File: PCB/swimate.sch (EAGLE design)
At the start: 46 parts, among them IC1 LPC11U24, T1 BSS84, T2 BSS84, U1 USD-SOCKETNEW, U5 DS3231MZ/V+T, U6 MAX1595EUA33+, U7 MAX1811ESA-T, U8 MAX16054AZT+T, U9 HC_05, Y1 12.000MHz

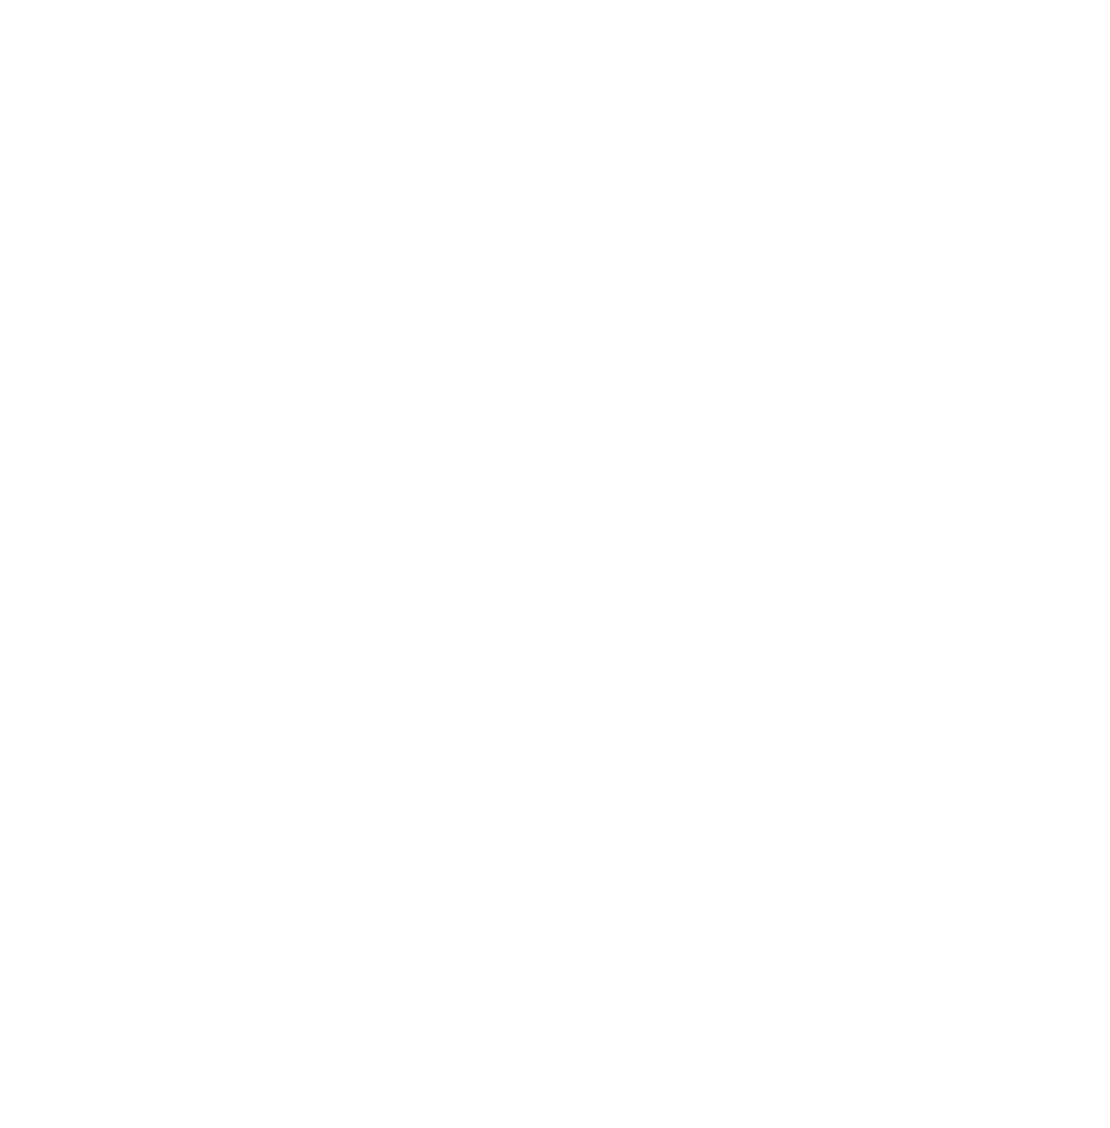
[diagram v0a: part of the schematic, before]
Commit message: Added dispaly
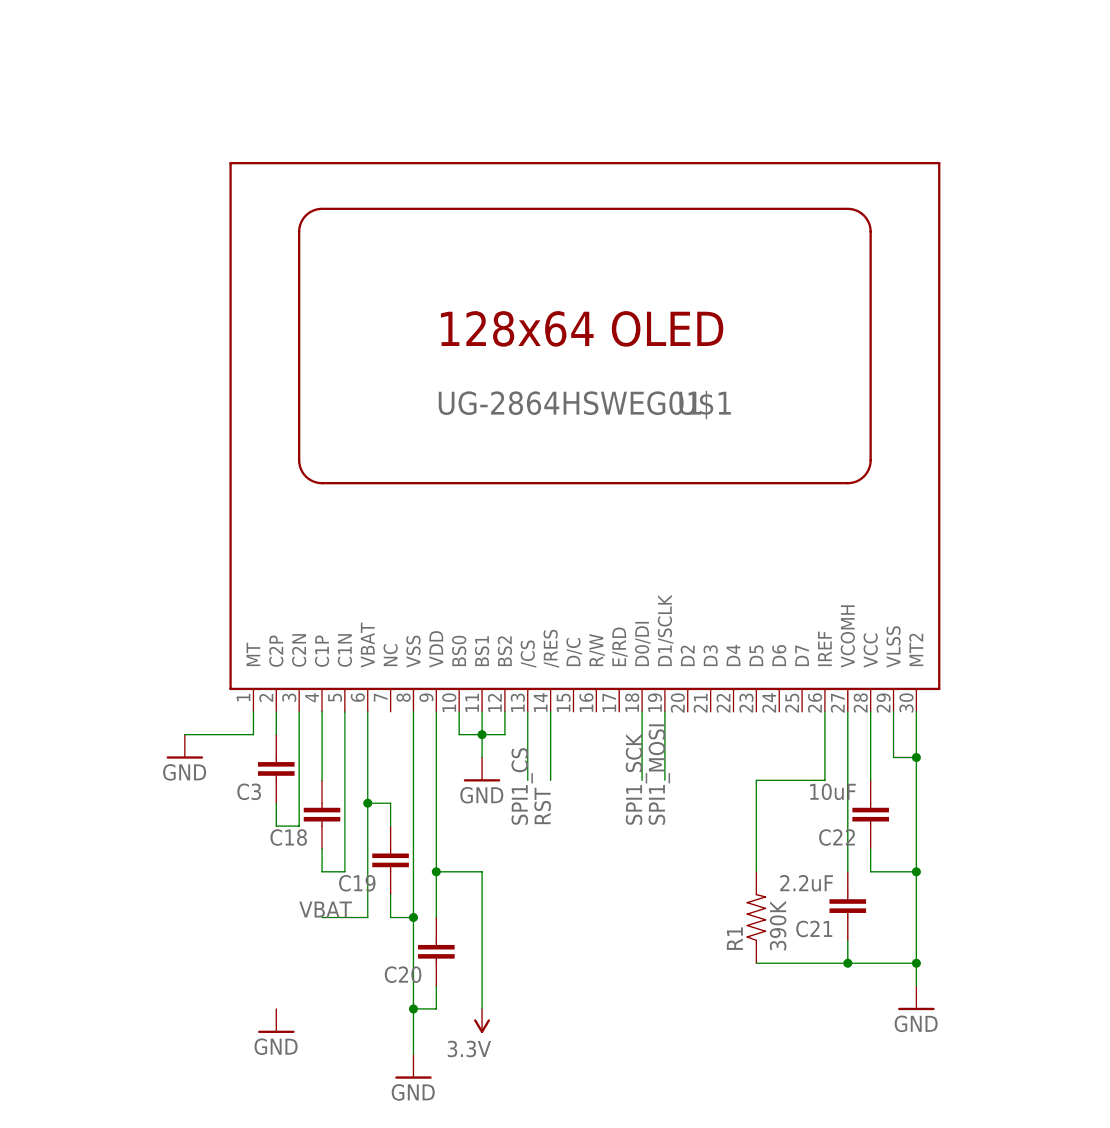
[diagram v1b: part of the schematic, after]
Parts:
- added C18, C19, C20, C3: (no value), SparkFun-Capacitors:CAP0805
- added C21: 2.2uF, SparkFun-Capacitors:CAP0805
- added C22: 10uF, SparkFun-Capacitors:CAP0805
- added R1: 390K, SparkFun-Passives:RESISTOR0805-RES
- added U$1: UG-2864HSWEG01, adafruit:UG-2864HSWEG01
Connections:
- new net N$2: C18.1, U$1.C1N
- new net N$25: C3.2, U$1.C2P
- new net N$26: C22.2, U$1.VCC
- new net N$27: C3.1, U$1.C2N
- new net N$28: C21.2, U$1.VCOMH
- new net N$29: C18.2, U$1.C1P
- new net N$3: R1.2, U$1.IREF
- new net SPI1_CS: U$1./CS
- new net SPI1_MOSI: U$1.D1/SCLK
- new net SPI1_SCK: U$1.D0/DI
- net 3.3V: now also C20.2, U$1.VDD
- net GND: now also C19.1, C20.1, C21.1, C22.1, R1.1, U$1.BS0, U$1.BS1, U$1.BS2, U$1.MT, U$1.MT2, U$1.VLSS, U$1.VSS
- net RST: now also U$1./RES
- net VBAT: now also C19.2, U$1.VBAT
